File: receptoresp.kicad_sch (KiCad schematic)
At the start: 2 parts

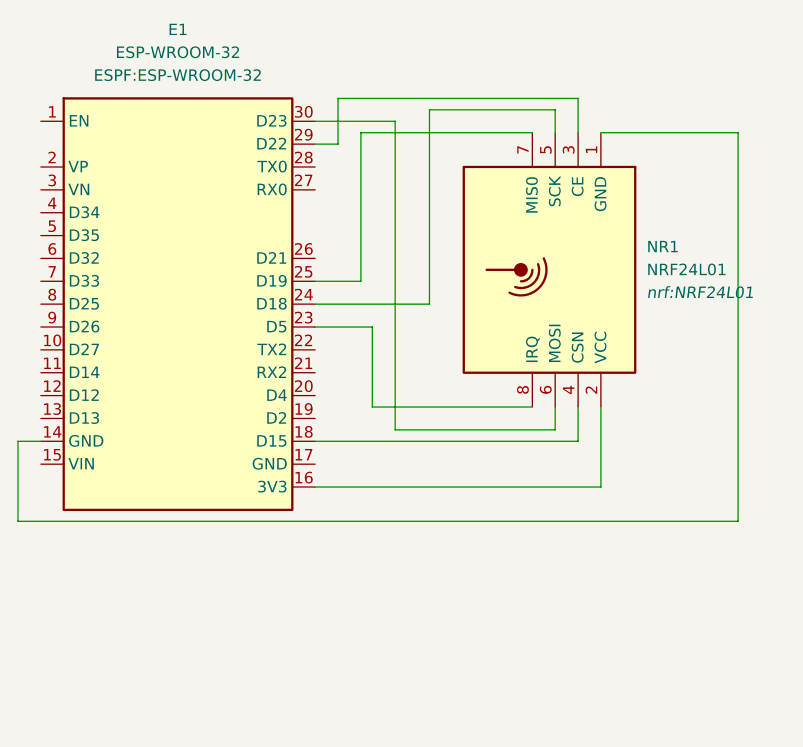
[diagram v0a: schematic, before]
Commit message: capacitor colocado para o modulo nrf
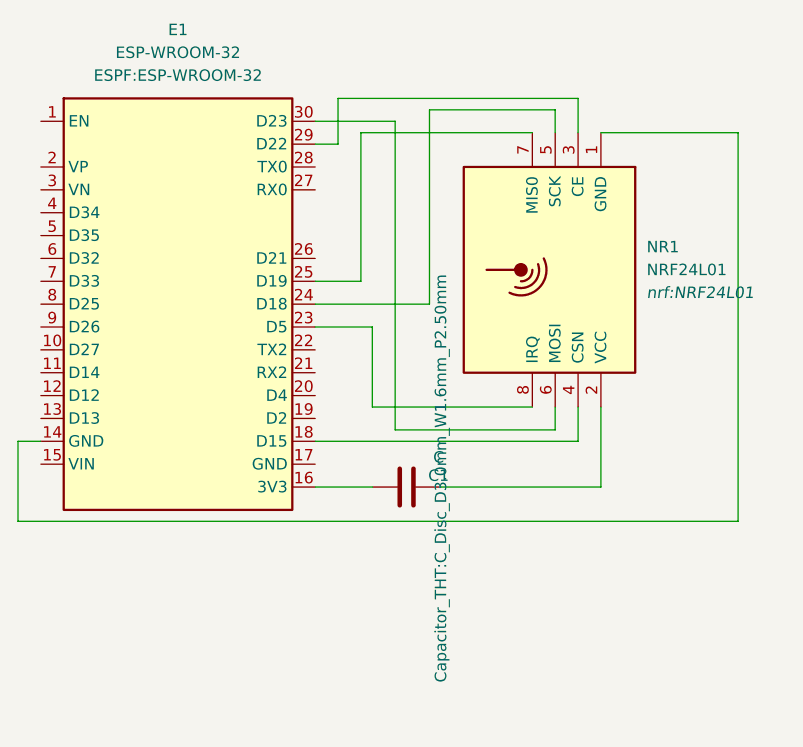
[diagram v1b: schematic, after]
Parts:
- added C1: C, Capacitor_THT:C_Disc_D3.0mm_W1.6mm_P2.50mm, symbol Device:C
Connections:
- net at NR1.2 (VCC): now also C1.2; no longer E1.16 (3V3)
- new net: C1.1, E1.16 (3V3)
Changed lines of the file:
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@@
 (kicad_sch
-	(version 20250114)
+	(version 20260306)
 	(generator "eeschema")
-	(generator_version "9.0")
+	(generator_version "10.0")
 	(paper "A4")
 	(wire
@@
 	(wire
 		(pts
+			(xy 167.64 93.98) (xy 173.99 93.98)
+		)
+		(stroke
+			(width 0)
+			(type default)
+		)
+	)
+	(wire
+		(pts
 			(xy 214.63 54.61) (xy 214.63 97.79)
 		)
@@
 	(wire
 		(pts
+			(xy 181.61 93.98) (xy 199.39 93.98)
+		)
+		(stroke
+			(width 0)
+			(type default)
+		)
+	)
+	(wire
+		(pts
 			(xy 172.72 71.12) (xy 167.64 71.12)
 		)
@@
 		(pts
 			(xy 196.85 50.8) (xy 196.85 54.61)
-		)
-		(stroke
-			(width 0)
-			(type default)
-		)
-	)
-	(wire
-		(pts
-			(xy 199.39 93.98) (xy 167.64 93.98)
 		)
 		(stroke
@@
 		(at 186.69 69.85 270)
 		(unit 1)
+		(body_style 1)
 		(exclude_from_sim no)
 		(in_bom yes)
 		(on_board yes)
+		(in_pos_files yes)
 		(dnp no)
 		(fields_autoplaced yes)
 		(property "Reference" "NR1"
 			(at 204.47 67.3099 90)
+			(show_name no)
+			(do_not_autoplace no)
 			(effects
 				(font
@@
 		(property "Value" "NRF24L01"
 			(at 204.47 69.8499 90)
+			(show_name no)
+			(do_not_autoplace no)
 			(effects
 				(font
@@
 		(property "Footprint" "nrf:NRF24L01"
 			(at 204.47 72.3899 90)
+			(show_name no)
+			(do_not_autoplace no)
 			(effects
 				(font
@@
 		(property "Datasheet" ""
 			(at 189.23 69.85 0)
-			(effects
-				(font
-					(size 1.27 1.27)
-				)
-				(hide yes)
+			(hide yes)
+			(show_name no)
+			(do_not_autoplace no)
+			(effects
+				(font
+					(size 1.27 1.27)
+				)
 			)
 		)
 		(property "Description" ""
 			(at 186.69 69.85 0)
-			(effects
-				(font
-					(size 1.27 1.27)
-				)
-				(hide yes)
+			(hide yes)
+			(show_name no)
+			(do_not_autoplace no)
+			(effects
+				(font
+					(size 1.27 1.27)
+				)
 			)
 		)
@@
 		)
 		(instances
-			(project ""
+			(project "receptoresp"
 				(path "/0e9bc2b5-e815-4e07-adb4-97dfc13169a1"
 					(reference "NR1")
@@
 		(at 152.4 76.2 0)
 		(unit 1)
+		(body_style 1)
 		(exclude_from_sim no)
 		(in_bom yes)
 		(on_board yes)
+		(in_pos_files yes)
 		(dnp no)
 		(fields_autoplaced yes)
 		(property "Reference" "E1"
 			(at 152.4 43.18 0)
+			(show_name no)
+			(do_not_autoplace no)
 			(effects
 				(font
@@
 		(property "Value" "ESP-WROOM-32"
 			(at 152.4 45.72 0)
+			(show_name no)
+			(do_not_autoplace no)
 			(effects
 				(font
@@
 		(property "Footprint" "ESPF:ESP-WROOM-32"
 			(at 152.4 48.26 0)
+			(show_name no)
+			(do_not_autoplace no)
 			(effects
 				(font
@@
 		(property "Datasheet" ""
 			(at 118.11 92.964 0)
-			(effects
-				(font
-					(size 1.27 1.27)
-				)
-				(hide yes)
+			(hide yes)
+			(show_name no)
+			(do_not_autoplace no)
+			(effects
+				(font
+					(size 1.27 1.27)
+				)
 			)
 		)
 		(property "Description" ""
 			(at 152.4 76.2 0)
-			(effects
-				(font
-					(size 1.27 1.27)
-				)
-				(hide yes)
+			(hide yes)
+			(show_name no)
+			(do_not_autoplace no)
+			(effects
+				(font
+					(size 1.27 1.27)
+				)
 			)
 		)
@@
 		)
 		(instances
-			(project ""
+			(project "receptoresp"
 				(path "/0e9bc2b5-e815-4e07-adb4-97dfc13169a1"
 					(reference "E1")
 					(unit 1)
 				)
+			)
+		)
+	)
+	(symbol
+		(lib_id "Device:C")
+		(at 177.8 93.98 90)
+		(unit 1)
+		(body_style 1)
+		(exclude_from_sim no)
+		(in_bom yes)
+		(on_board yes)
+		(in_pos_files yes)
+		(dnp no)
+		(property "Reference" "C1"
+			(at 181.356 92.71 90)
+			(show_name no)
+			(do_not_autoplace no)
+			(effects
+				(font
+					(size 1.27 1.27)
+				)
+			)
+		)
+		(property "Value" "C"
+			(at 181.356 90.678 90)
+			(show_name no)
+			(do_not_autoplace no)
+			(effects
+				(font
+					(size 1.27 1.27)
+				)
+			)
+		)
+		(property "Footprint" "Capacitor_THT:C_Disc_D3.0mm_W1.6mm_P2.50mm"
+			(at 181.61 93.0148 0)
+			(show_name no)
+			(do_not_autoplace no)
+			(effects
+				(font
+					(size 1.27 1.27)
+				)
+			)
+		)
+		(property "Datasheet" ""
+			(at 177.8 93.98 0)
+			(hide yes)
+			(show_name no)
+			(do_not_autoplace no)
+			(effects
+				(font
+					(size 1.27 1.27)
+				)
+			)
+		)
+		(property "Description" "Unpolarized capacitor"
+			(at 177.8 93.98 0)
+			(hide yes)
+			(show_name no)
+			(do_not_autoplace no)
+			(effects
+				(font
+					(size 1.27 1.27)
+				)
+			)
+		)
+		(pin "1"
+		)
+		(pin "2"
+		)
+		(instances
+			(project "receptoresp"
+				(path "/0e9bc2b5-e815-4e07-adb4-97dfc13169a1"
+					(reference "C1")
+					(unit 1)
+				)
